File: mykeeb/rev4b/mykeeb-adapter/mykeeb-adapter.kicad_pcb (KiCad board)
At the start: 2 copper layers, 128 x 121.7 mm, 33 parts, among them J10 Conn_01x04_Female, J11 Conn_01x05, J12 Conn_01x04_Female, J2 Conn_01x02, J3 Conn_02x07_Odd_Even, J8 Conn_01x04_Female, J9 Conn_01x04_Female, K40 KEYSW, K41 KEYSW, K42 KEYSW, K43 KEYSW, K44 KEYSW, K45 KEYSW, K46 KEYSW, SW1 SW_Push, U1 ProMicro

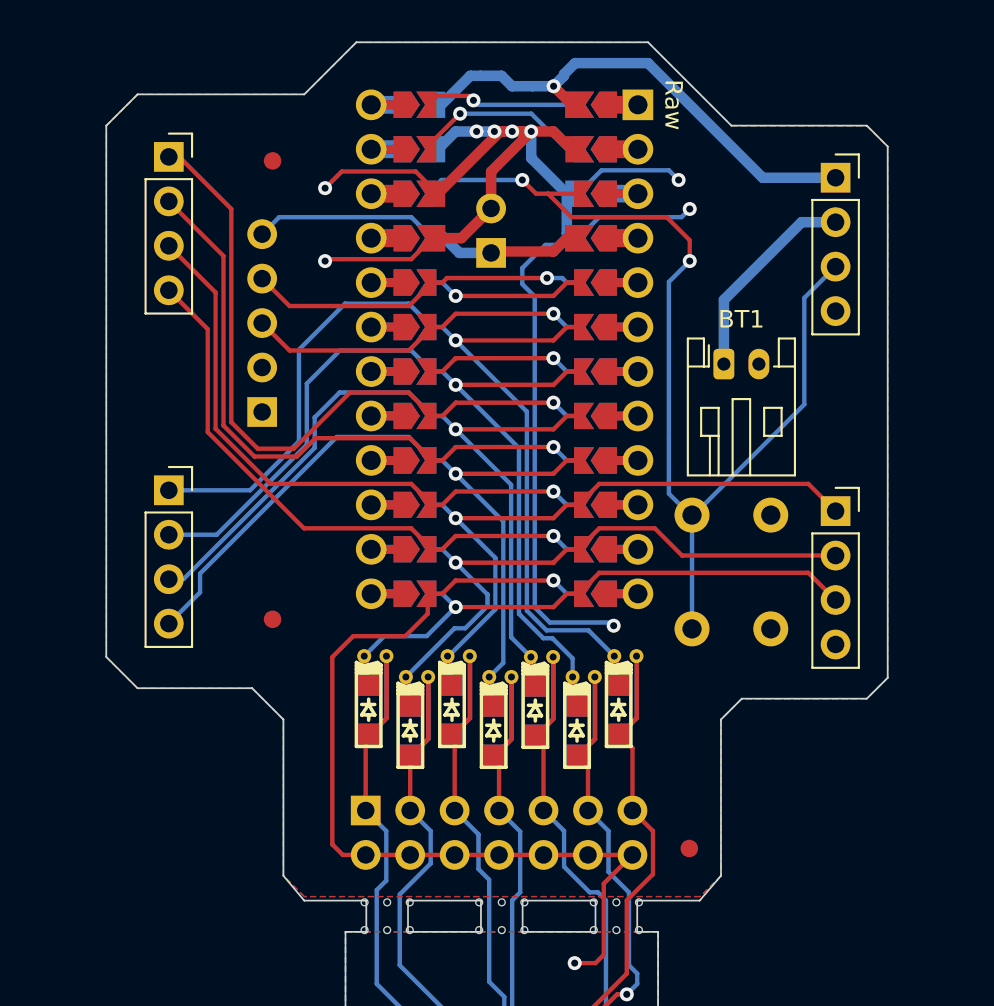
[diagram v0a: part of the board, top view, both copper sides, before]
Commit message: udpate
Signed-off-by: Maximilian Huber <gh@maxhbr.de>
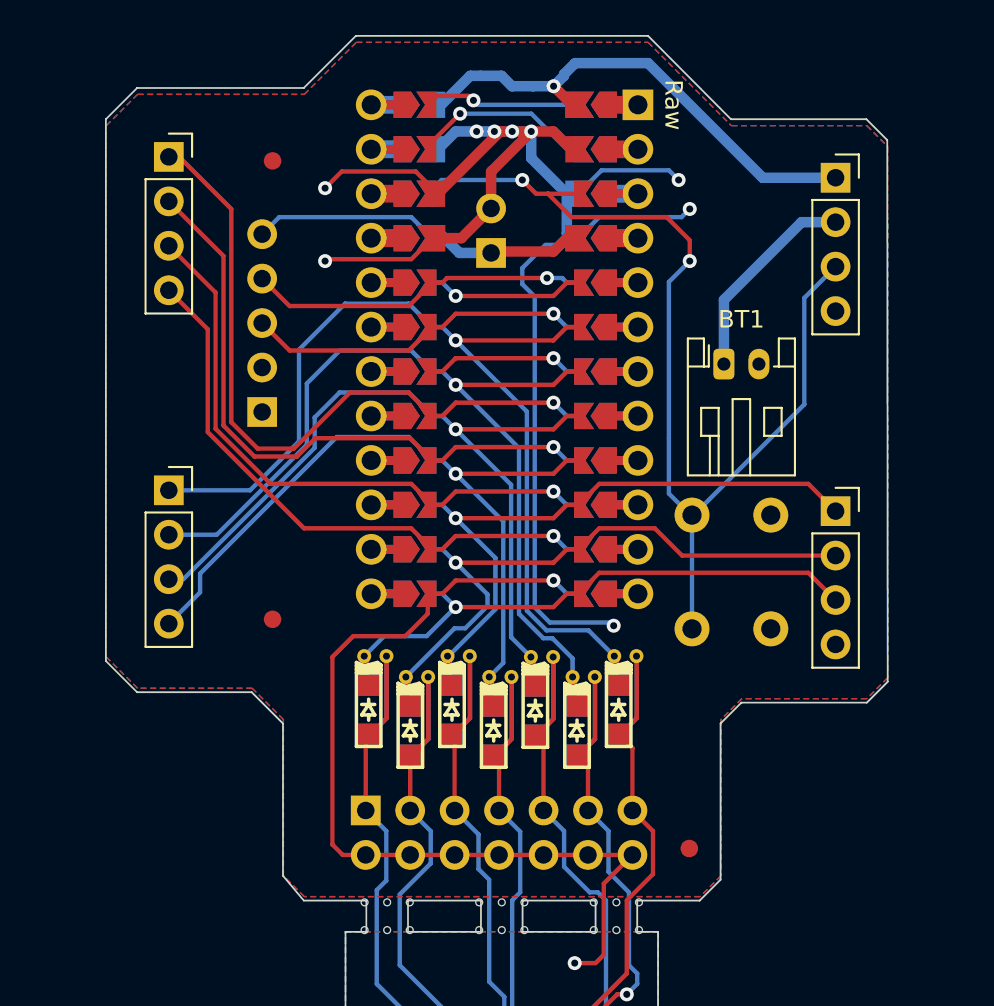
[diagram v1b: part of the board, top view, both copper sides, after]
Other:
- board size 128 x 121.7 mm -> 128 x 122 mm
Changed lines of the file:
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@@
   (gr_poly
     (pts
-      (xy 107.181237 39.657808)
-      (xy 114.920306 39.657808)
-      (xy 116.110932 40.848434)
-      (xy 116.110932 71.209397)
-      (xy 114.920306 72.400023)
-      (xy 107.77655 72.400023)
-      (xy 106.585924 73.590649)
-      (xy 106.585924 82.520344)
+      (xy 107.15634 39.290658)
+      (xy 114.895409 39.290658)
+      (xy 116.086035 40.481284)
+      (xy 116.110932 71.43756)
+      (xy 114.920306 72.628186)
+      (xy 107.751653 72.628186)
+      (xy 106.561027 73.818812)
+      (xy 106.561027 82.748507)
       (xy 105.370401 83.939133)
       (xy 101.798523 83.939133)
@@
       (xy 86.320385 85.725072)
       (xy 86.320385 83.939133)
-      (xy 82.773404 83.939133)
-      (xy 81.582778 82.520344)
-      (xy 81.582778 73.590649)
-      (xy 79.796839 71.80471)
-      (xy 73.248396 71.80471)
-      (xy 71.462457 70.018771)
-      (xy 71.462457 39.657808)
-      (xy 73.248396 37.871869)
-      (xy 82.773404 37.871869)
-      (xy 85.749969 34.895304)
-      (xy 102.418733 34.895304)
+      (xy 82.748507 83.939133)
+      (xy 81.557881 82.520344)
+      (xy 81.557881 73.818812)
+      (xy 79.771942 72.032873)
+      (xy 73.223499 72.032873)
+      (xy 71.43756 70.246934)
+      (xy 71.43756 39.290658)
+      (xy 73.223499 37.504719)
+      (xy 82.748507 37.504719)
+      (xy 85.725072 34.528154)
+      (xy 102.418733 34.528154)
     ) (layer "Edge.Cuts") (width 0.1) (fill none))
   (gr_circle (center 147.042311 129.182921) (end 148.542311 129.182921) (layer "User.1") (width 0.15) (fill none))
   (gr_circle (center 98.226645 110.132905) (end 99.726645 110.132905) (layer "User.1") (width 0.15) (fill none))
   (gr_circle (center 70.842247 116.086035) (end 72.342247 116.086035) (layer "User.1") (width 0.15) (fill none))
+  (gr_poly
+    (pts
+      (xy 113.704783 57.745361)
+      (xy 113.704783 53.57817)
+      (xy 116.086035 52.387544)
+      (xy 116.086035 58.935987)
+    ) (layer "User.4") (width 0.15) (fill solid))
+  (gr_poly
+    (pts
+      (xy 74.414125 39.290658)
+      (xy 73.223499 40.481284)
+      (xy 71.43756 41.67191)
+      (xy 71.43756 39.290658)
+      (xy 73.223499 37.504719)
+      (xy 75.604751 37.504719)
+    ) (layer "User.4") (width 0.15) (fill solid))
+  (gr_poly
+    (pts
+      (xy 73.223499 69.056308)
+      (xy 74.414125 70.246934)
+      (xy 75.604751 72.032873)
+      (xy 73.223499 72.032873)
+      (xy 71.43756 70.246934)
+      (xy 71.43756 67.865682)
+    ) (layer "User.4") (width 0.15) (fill solid))
   (gr_poly
     (pts
@@
       (xy 165.497014 114.300096)
     ) (layer "User.4") (width 0.15) (fill solid))
+  (gr_poly
+    (pts
+      (xy 73.818812 52.982857)
+      (xy 73.818812 57.150048)
+      (xy 71.43756 58.340674)
+      (xy 71.43756 51.792231)
+    ) (layer "User.4") (width 0.15) (fill solid))
   (gr_line locked (start 91.709836 94.343738) (end 77.739074 94.343738) (layer "User.5") (width 0.25))
